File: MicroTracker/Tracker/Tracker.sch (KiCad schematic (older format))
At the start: 0 parts

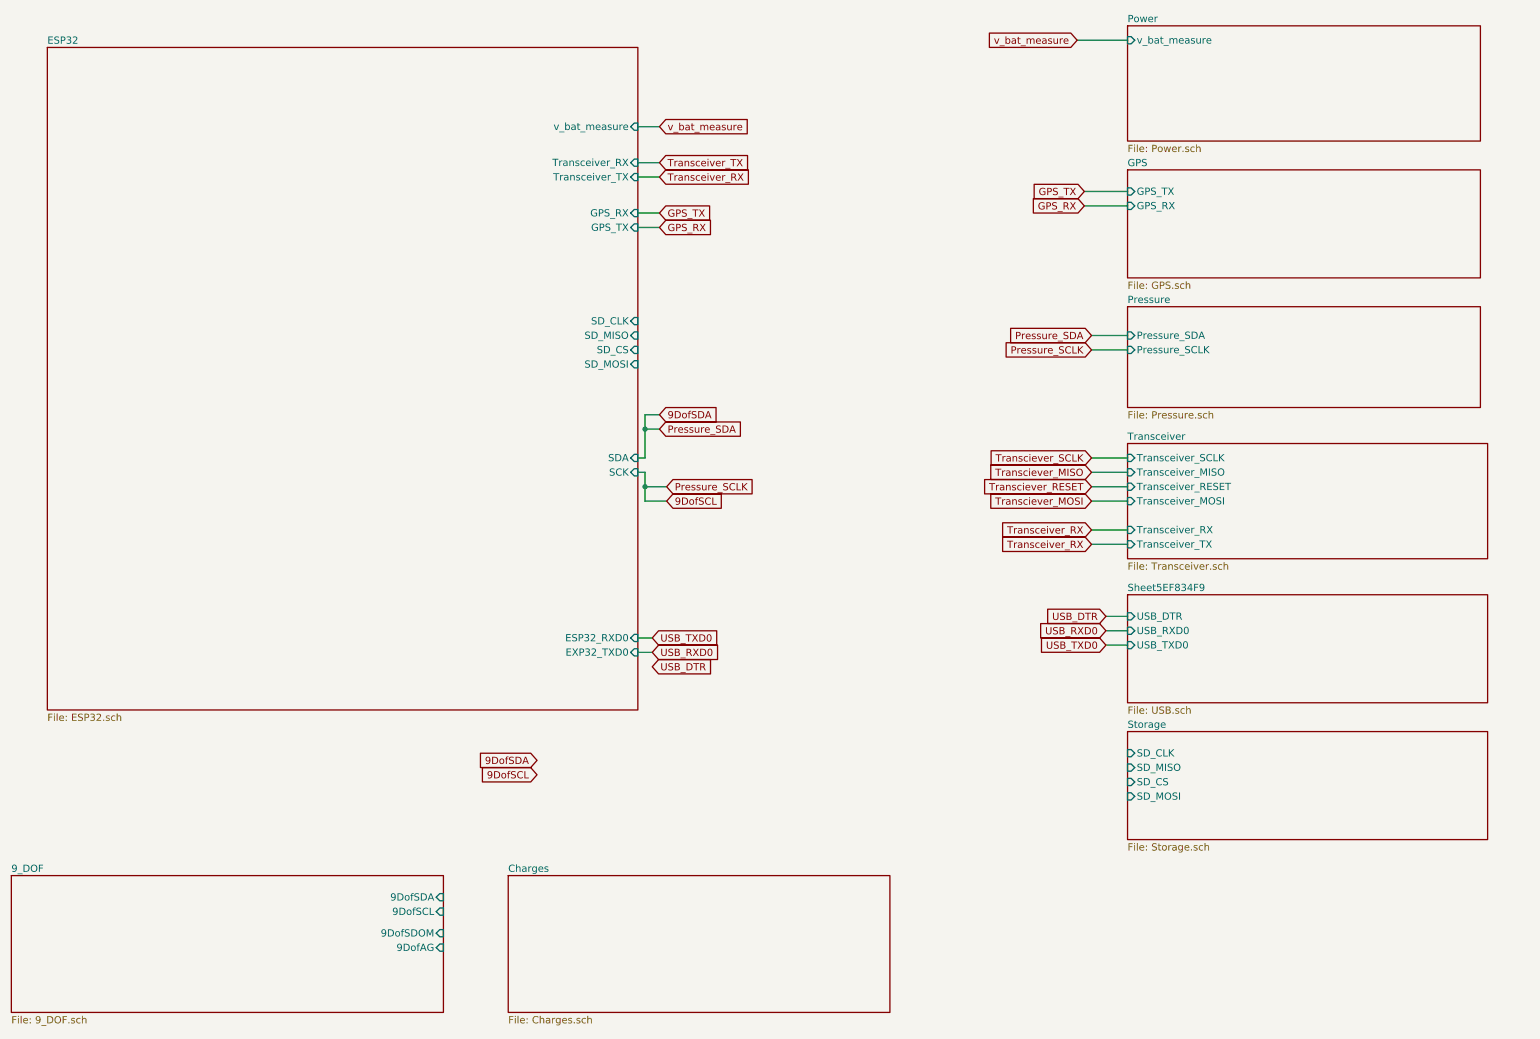
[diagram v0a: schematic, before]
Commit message: added connections
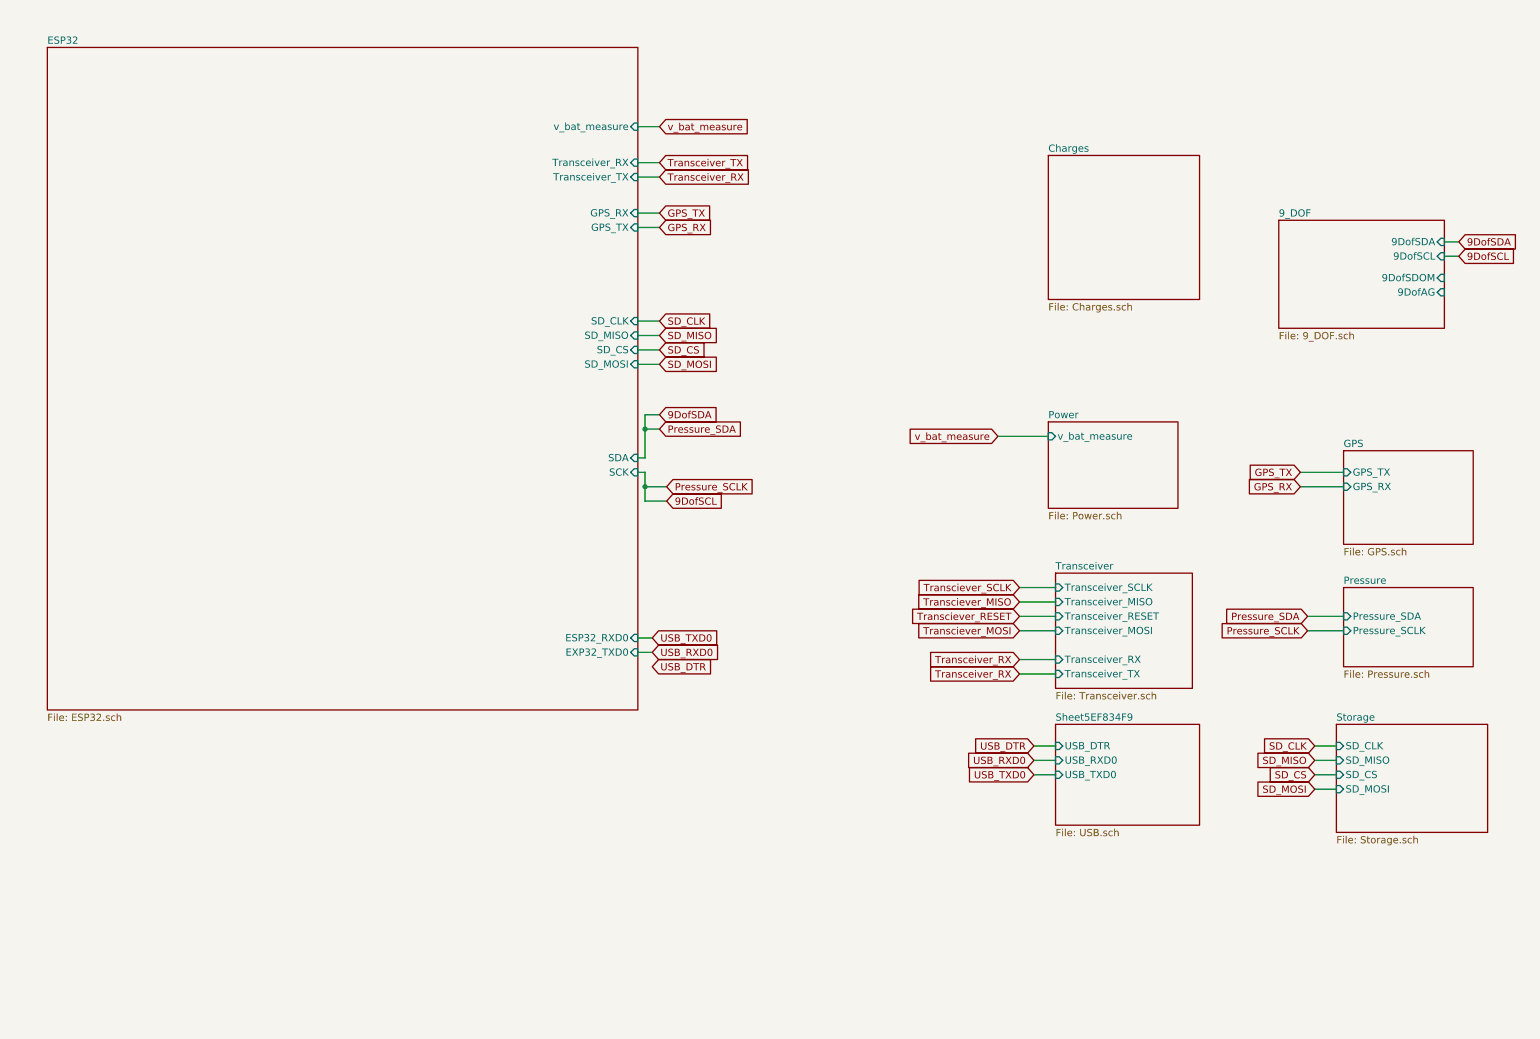
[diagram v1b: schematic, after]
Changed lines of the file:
@@
 $EndDescr
 $Sheet
-S 8350 700  2450 800
+S 7800 3450 900  600
 U 5EF7F21E
 F0 "Power" 50
 F1 "Power.sch" 50
-F2 "v_bat_measure" I L 8350 800 50
-$EndSheet
-$Sheet
-S 8350 1700 2450 750
+F2 "v_bat_measure" I L 7800 3550 50
+$EndSheet
+$Sheet
+S 9850 3650 900  650
 U 5EF7F258
 F0 "GPS" 50
 F1 "GPS.sch" 50
-F2 "GPS_TX" I L 8350 1850 50
-F3 "GPS_RX" I L 8350 1950 50
-$EndSheet
-$Sheet
-S 8350 2650 2450 700
+F2 "GPS_TX" I L 9850 3800 50
+F3 "GPS_RX" I L 9850 3900 50
+$EndSheet
+$Sheet
+S 9850 4600 900  550
 U 5EF7F2B3
 F0 "Pressure" 50
 F1 "Pressure.sch" 50
-F2 "Pressure_SDA" I L 8350 2850 50
-F3 "Pressure_SCLK" I L 8350 2950 50
-$EndSheet
-$Sheet
-S 8350 3600 2500 800
+F2 "Pressure_SDA" I L 9850 4800 50
+F3 "Pressure_SCLK" I L 9850 4900 50
+$EndSheet
+$Sheet
+S 7850 4500 950  800
 U 5EF7F30A
 F0 "Transceiver" 50
 F1 "Transceiver.sch" 50
-F2 "Transceiver_SCLK" I L 8350 3700 50
-F3 "Transceiver_MISO" I L 8350 3800 50
-F4 "Transceiver_RESET" I L 8350 3900 50
-F5 "Transceiver_MOSI" I L 8350 4000 50
-F6 "Transceiver_TX" I L 8350 4300 50
-F7 "Transceiver_RX" I L 8350 4200 50
+F2 "Transceiver_SCLK" I L 7850 4600 50
+F3 "Transceiver_MISO" I L 7850 4700 50
+F4 "Transceiver_RESET" I L 7850 4800 50
+F5 "Transceiver_MOSI" I L 7850 4900 50
+F6 "Transceiver_TX" I L 7850 5200 50
+F7 "Transceiver_RX" I L 7850 5100 50
 $EndSheet
 $Sheet
@@
 $EndSheet
 $Sheet
-S 8350 4650 2500 750
+S 7850 5550 1000 700
 U 5EF834FA
 F0 "Sheet5EF834F9" 50
 F1 "USB.sch" 50
-F2 "USB_DTR" I L 8350 4800 50
-F3 "USB_RXD0" I L 8350 4900 50
-F4 "USB_TXD0" I L 8350 5000 50
-$EndSheet
-Text GLabel 8100 2850 0    50   Input ~ 0
+F2 "USB_DTR" I L 7850 5700 50
+F3 "USB_RXD0" I L 7850 5800 50
+F4 "USB_TXD0" I L 7850 5900 50
+$EndSheet
+Text GLabel 9600 4800 0    50   Input ~ 0
 Pressure_SDA
-Text GLabel 8100 2950 0    50   Input ~ 0
+Text GLabel 9600 4900 0    50   Input ~ 0
 Pressure_SCLK
-Text GLabel 8100 3700 0    50   Input ~ 0
+Text GLabel 7600 4600 0    50   Input ~ 0
 Transciever_SCLK
-Text GLabel 8100 3800 0    50   Input ~ 0
+Text GLabel 7600 4700 0    50   Input ~ 0
 Transciever_MISO
-Text GLabel 8100 3900 0    50   Input ~ 0
+Text GLabel 7600 4800 0    50   Input ~ 0
 Transciever_RESET
-Text GLabel 8100 4000 0    50   Input ~ 0
+Text GLabel 7600 4900 0    50   Input ~ 0
 Transciever_MOSI
 Wire Wire Line
-	8100 3700 8350 3700
-Wire Wire Line
-	8100 3800 8350 3800
-Wire Wire Line
-	8100 3900 8350 3900
-Wire Wire Line
-	8100 4000 8350 4000
-Text GLabel 8050 1850 0    50   Input ~ 0
+	7600 4600 7850 4600
+Wire Wire Line
+	7600 4700 7850 4700
+Wire Wire Line
+	7600 4800 7850 4800
+Wire Wire Line
+	7600 4900 7850 4900
+Text GLabel 9550 3800 0    50   Input ~ 0
 GPS_TX
-Text GLabel 8050 1950 0    50   Input ~ 0
+Text GLabel 9550 3900 0    50   Input ~ 0
 GPS_RX
 Wire Wire Line
-	8050 1850 8350 1850
-Wire Wire Line
-	8050 1950 8350 1950
-Text GLabel 8000 800  0    50   Input ~ 0
+	9550 3800 9850 3800
+Wire Wire Line
+	9550 3900 9850 3900
+Text GLabel 7450 3550 0    50   Input ~ 0
 v_bat_measure
 Wire Wire Line
-	8000 800  8350 800
-Wire Wire Line
-	8100 2850 8350 2850
-Wire Wire Line
-	8100 2950 8350 2950
+	7450 3550 7800 3550
+Wire Wire Line
+	9600 4800 9850 4800
+Wire Wire Line
+	9600 4900 9850 4900
 Text GLabel 5100 3500 2    50   Input ~ 0
 Pressure_SDA
@@
 v_bat_measure
 $Sheet
-S 8350 5600 2500 750
+S 9800 5550 1050 750
 U 5EF91B46
 F0 "Storage" 50
 F1 "Storage.sch" 50
-F2 "SD_CLK" I L 8350 5750 50
-F3 "SD_MISO" I L 8350 5850 50
-F4 "SD_CS" I L 8350 5950 50
-F5 "SD_MOSI" I L 8350 6050 50
-$EndSheet
-Text GLabel 8200 4900 0    50   Input ~ 0
+F2 "SD_CLK" I L 9800 5700 50
+F3 "SD_MISO" I L 9800 5800 50
+F4 "SD_CS" I L 9800 5900 50
+F5 "SD_MOSI" I L 9800 6000 50
+$EndSheet
+Text GLabel 7700 5800 0    50   Input ~ 0
 USB_RXD0
-Text GLabel 8200 4800 0    50   Input ~ 0
+Text GLabel 7700 5700 0    50   Input ~ 0
 USB_DTR
-Text GLabel 8200 5000 0    50   Input ~ 0
+Text GLabel 7700 5900 0    50   Input ~ 0
 USB_TXD0
 Text GLabel 5050 5050 2    50   Input ~ 0
@@
 USB_TXD0
 Wire Wire Line
-	8200 4800 8350 4800
-Wire Wire Line
-	8200 4900 8350 4900
-Wire Wire Line
-	8200 5000 8350 5000
+	7700 5700 7850 5700
+Wire Wire Line
+	7700 5800 7850 5800
+Wire Wire Line
+	7700 5900 7850 5900
 Wire Wire Line
 	5050 4950 4950 4950
 Wire Wire Line
 	4950 5050 5050 5050
-Text GLabel 8100 4200 0    50   Input ~ 0
+Text GLabel 7600 5100 0    50   Input ~ 0
 Transceiver_RX
-Text GLabel 8100 4300 0    50   Input ~ 0
+Text GLabel 7600 5200 0    50   Input ~ 0
 Transceiver_RX
 Wire Wire Line
-	8100 4200 8350 4200
-Wire Wire Line
-	8100 4300 8350 4300
+	7600 5100 7850 5100
+Wire Wire Line
+	7600 5200 7850 5200
 Text GLabel 5100 1750 2    50   Input ~ 0
 Transceiver_RX
@@
 Transceiver_TX
 $Sheet
-S 4050 6600 2650 950
+S 7800 1600 1050 1000
 U 5EFA735D
 F0 "Charges" 50
@@
 	4950 2100 5100 2100
 $Sheet
-S 600  6600 3000 950
+S 9400 2050 1150 750
 U 5F07F54B
 F0 "9_DOF" 50
 F1 "9_DOF.sch" 50
-F2 "9DofSDA" I R 3600 6750 50
-F3 "9DofSCL" I R 3600 6850 50
-F4 "9DofSDOM" I R 3600 7000 50
-F5 "9DofAG" I R 3600 7100 50
-$EndSheet
-Text GLabel 4250 5800 0    50   Input ~ 0
+F2 "9DofSDA" I R 10550 2200 50
+F3 "9DofSCL" I R 10550 2300 50
+F4 "9DofSDOM" I R 10550 2450 50
+F5 "9DofAG" I R 10550 2550 50
+$EndSheet
+Text GLabel 10650 2200 2    50   Input ~ 0
 9DofSDA
-Text GLabel 4250 5900 0    50   Input ~ 0
+Text GLabel 10650 2300 2    50   Input ~ 0
 9DofSCL
 Text GLabel 5100 3400 2    50   Input ~ 0
@@
 Wire Wire Line
 	5000 3900 5000 4000
+Text GLabel 9650 5700 0    50   Input ~ 0
+SD_CLK
+Text GLabel 9650 5800 0    50   Input ~ 0
+SD_MISO
+Text GLabel 9650 5900 0    50   Input ~ 0
+SD_CS
+Text GLabel 9650 6000 0    50   Input ~ 0
+SD_MOSI
+Wire Wire Line
+	9650 5700 9800 5700
+Wire Wire Line
+	9650 5800 9800 5800
+Wire Wire Line
+	9650 5900 9800 5900
+Wire Wire Line
+	9650 6000 9800 6000
+Text GLabel 5100 2750 2    50   Input ~ 0
+SD_CLK
+Text GLabel 5100 2850 2    50   Input ~ 0
+SD_MISO
+Text GLabel 5100 2950 2    50   Input ~ 0
+SD_CS
+Text GLabel 5100 3050 2    50   Input ~ 0
+SD_MOSI
+Wire Wire Line
+	4950 2750 5100 2750
+Wire Wire Line
+	4950 2850 5100 2850
+Wire Wire Line
+	4950 2950 5100 2950
+Wire Wire Line
+	4950 3050 5100 3050
+Wire Wire Line
+	10550 2200 10650 2200
+Wire Wire Line
+	10550 2300 10650 2300
 $EndSCHEMATC
